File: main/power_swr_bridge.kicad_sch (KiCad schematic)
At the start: 17 parts, among them J7 Conn_Coaxial

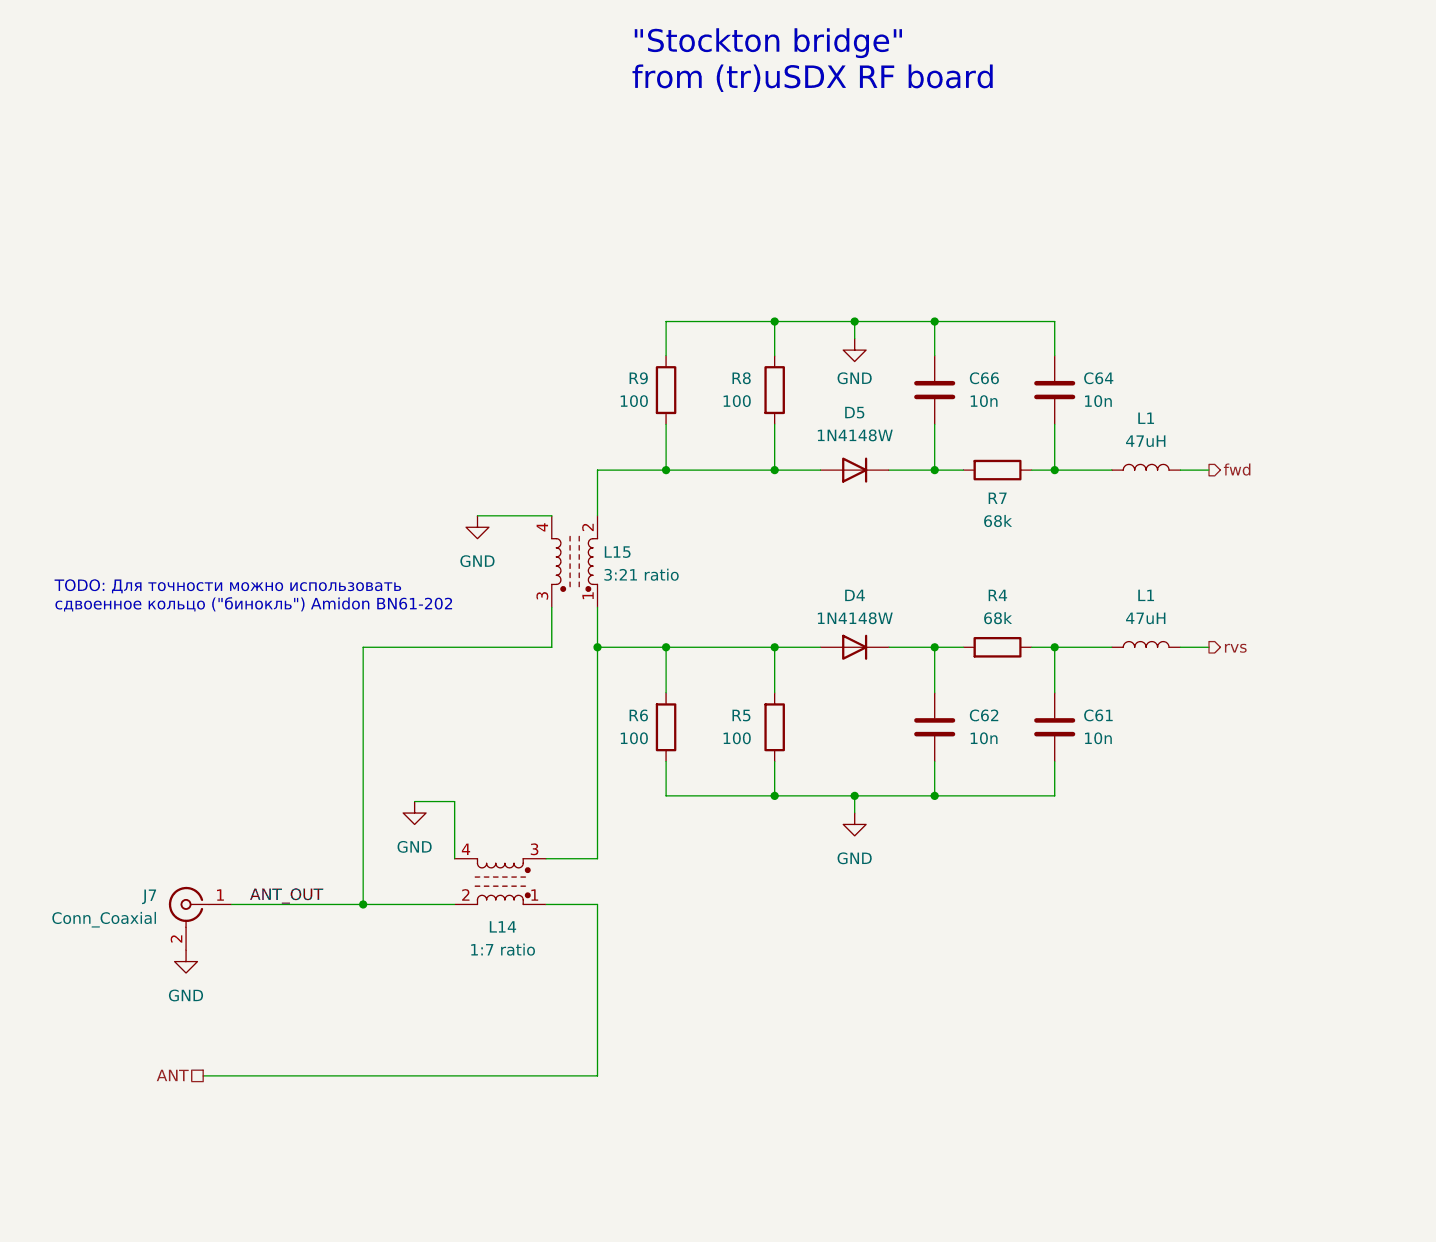
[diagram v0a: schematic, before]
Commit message: SWR meter circuit updated
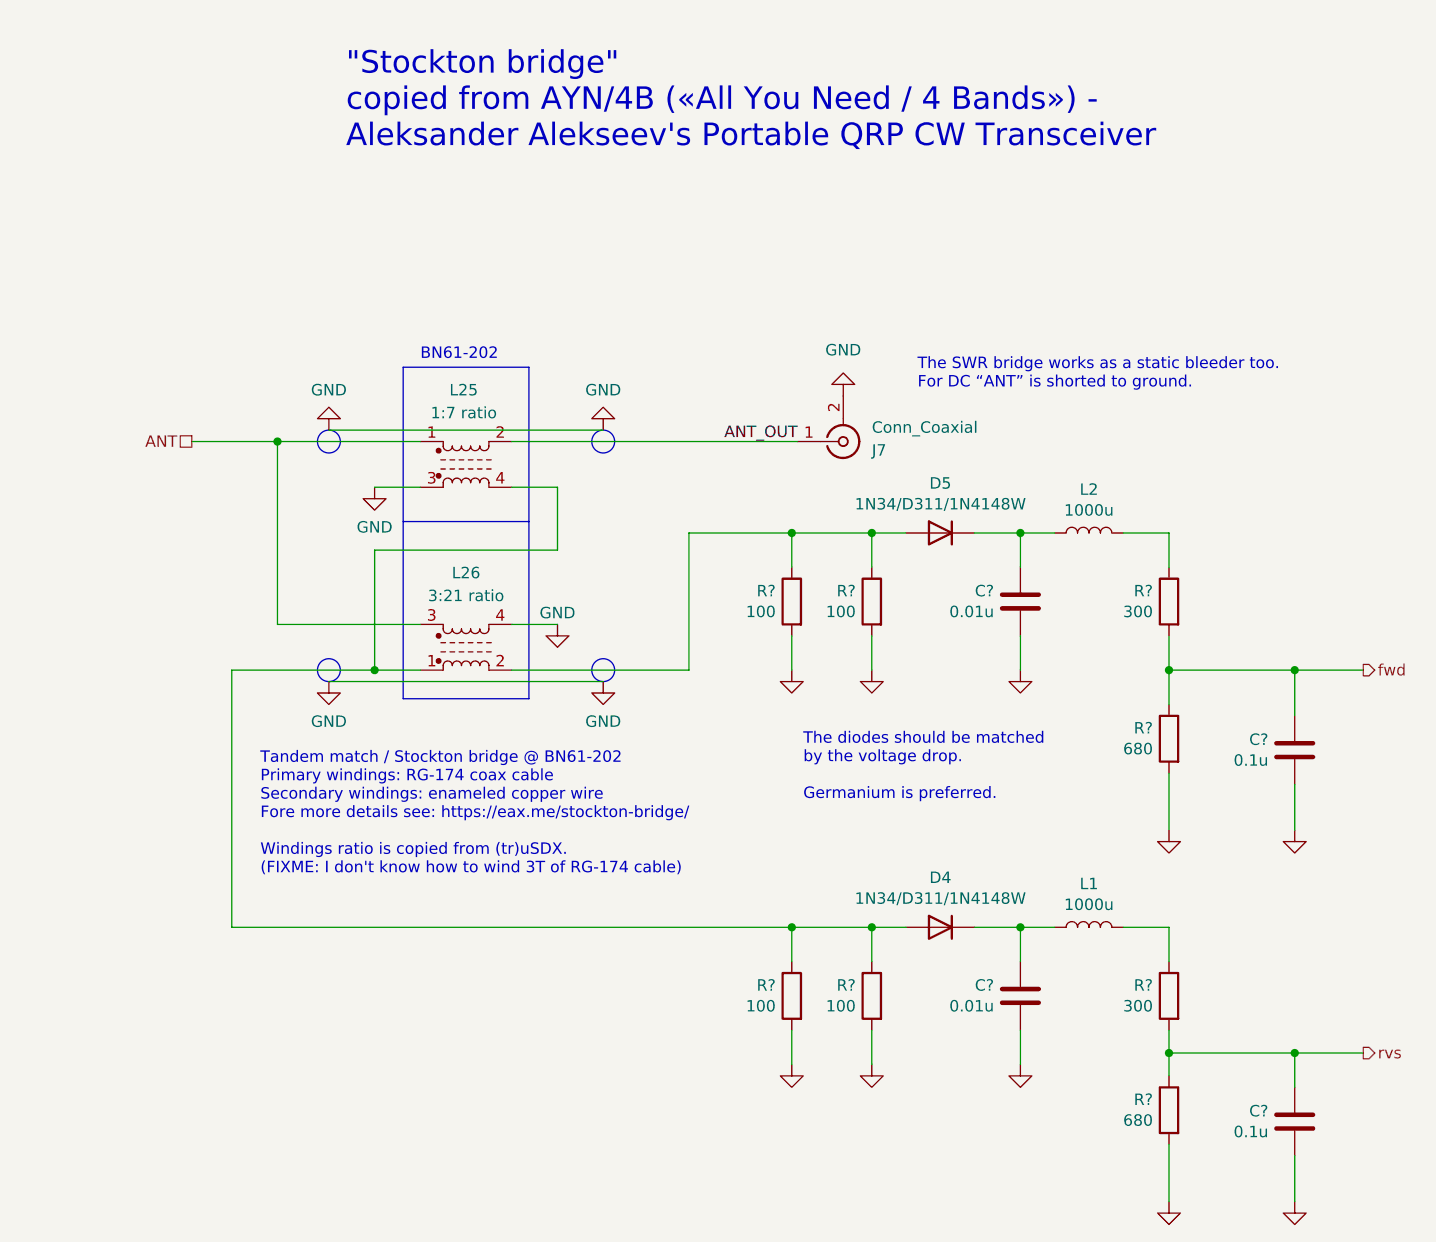
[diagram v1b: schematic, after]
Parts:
- removed C61, C62, C64, C66: 10n, symbol Device:C
- removed D4, D5: 1N4148W, Diode_SMD:D_SOD-123, symbol Diode:1N4148W
- removed L1 (x2): 47uH, symbol Device:L
- removed L14: 1:7 ratio, symbol Device:L_Ferrite_Coupled
- removed L15: 3:21 ratio, symbol Device:L_Ferrite_Coupled
- removed R4, R7: 68k, symbol Device:R
- removed R5, R6, R8, R9: 100, symbol Device:R
- added C? (x2): 0.1u, Capacitor_SMD:C_0805_2012Metric_Pad1.15x1.40mm_HandSolder, symbol Device:C
- added C? (x2): 0.01u, Capacitor_SMD:C_0805_2012Metric_Pad1.15x1.40mm_HandSolder, symbol Device:C
- added D4, D5: 1N34/D311/1N4148W, symbol Device:D
- added L1, L2: 1000u, Diode_THT:D_DO-41_SOD81_P2.54mm_Vertical_AnodeUp, symbol Device:L
- added L25: 1:7 ratio, symbol Device:L_Ferrite_Coupled
- added L26: 3:21 ratio, symbol Device:L_Ferrite_Coupled
- added R? (x4): 100, Resistor_SMD:R_0805_2012Metric_Pad1.15x1.40mm_HandSolder, symbol Device:R
- added R? (x2): 300, Resistor_SMD:R_0805_2012Metric_Pad1.15x1.40mm_HandSolder, symbol Device:R
- added R? (x2): 680, Resistor_SMD:R_0805_2012Metric_Pad1.15x1.40mm_HandSolder, symbol Device:R
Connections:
- net ANT: now also L25.1, L26.3
- net ANT_OUT: now also L25.2
- net GND: now also C?.2, C?.2, C?.2, C?.2, L25.3, L26.4, R?.2, R?.2, R?.2, R?.2, R?.2, R?.2
- net fwd: now also C?.1, R?.1, R?.2
- net rvs: now also C?.1, R?.1, R?.2
- new net: C?.1, D4.1 (K), L1.2
- new net: D4.2 (A), L25.4, L26.1, R?.1, R?.1
- new net: D5.2 (A), L26.2, R?.1, R?.1
- new net: L2.1, R?.1
- new net: C?.1, D5.1 (K), L2.2
- new net: L1.1, R?.1
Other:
- note added: ""Stockton bridge" copied from AYN/4B («All You Need / 4 Bands») - Aleksander Alekseev's Portable QRP CW Transceiver"
- note added: "BN61-202"
- note added: "Tandem match / Stockton bridge @ BN61-202 Primary windings: RG-174 coax cable Secondary windings: enameled copper wire Fore more details see: https://eax.me/stockton-bridge/ Windings ratio is copied from (tr)uSDX. (FIXME: I don't know how to wind 3T of RG-174 cable)"
- note added: "The SWR bridge works as a static bleeder too. For DC “ANT” is shorted to ground."
- note added: "The diodes should be matched by the voltage drop. Germanium is preferred."
- note removed: ""Stockton bridge" from (tr)uSDX RF board"
- note removed: "TODO: Для точности можно использовать сдвоенное кольцо ("бинокль") Amidon BN61-202"
- moved on the sheet: J7
